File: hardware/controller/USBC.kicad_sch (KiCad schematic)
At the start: 1 part, among them J1 Joystick

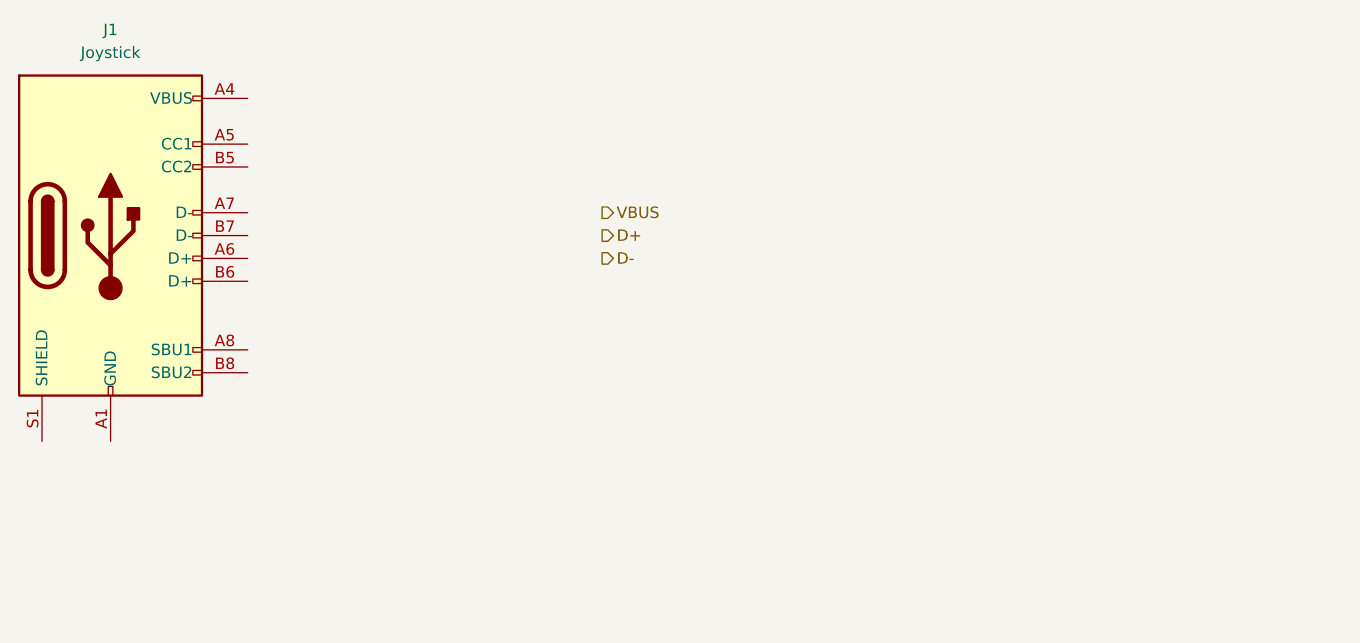
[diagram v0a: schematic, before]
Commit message: a
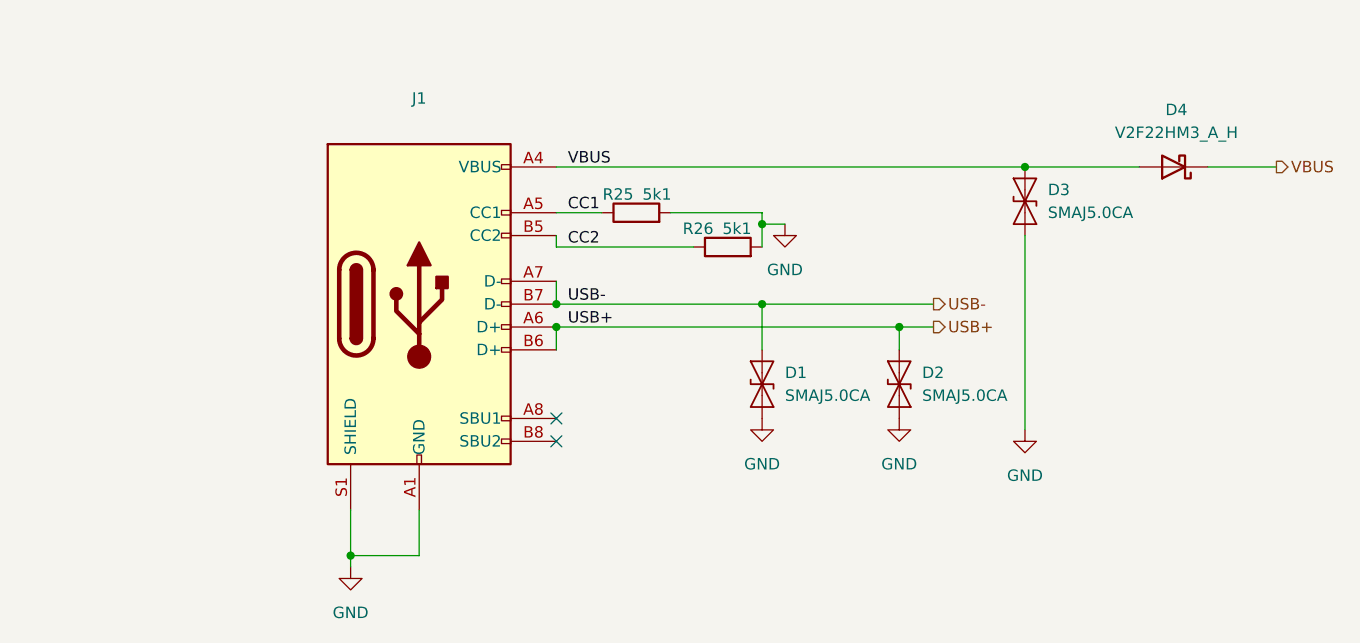
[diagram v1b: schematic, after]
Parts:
- added D1, D2, D3: SMAJ5.0CA, Diode_SMD:Infineon_SG-WLL-2-3_0.58x0.28_P0.36mm, symbol Diode:ESD131-B1-W0201
- added D4: V2F22HM3_A_H, Diode_SMD:D_SMA, symbol Diode:SS3150
- added R25, R26: 5k1, symbol Device:R
- J1: value Joystick -> ~
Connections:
- net VBUS: now also J1.A4 (VBUS), J1.A9 (VBUS), J1.B4 (VBUS), J1.B9 (VBUS), D3.2 (A2), D4.1 (K), D4.2 (A)
- net GND: now reaches J1.A1 (GND), J1.A12 (GND), J1.B1 (GND), J1.B12 (GND)
- net GND: now also J1.S1 (SHIELD), D1.1 (A1), D2.1 (A1), D3.1 (A1), R25.2, R26.2
- net CC1: now reaches J1.A5 (CC1)
- net CC1: now also R25.1
- net USB+: now reaches J1.A6 (D+)
- net USB+: now also J1.B6 (D+), D2.2 (A2)
- net USB-: now reaches J1.A7 (D-)
- net USB-: now also J1.B7 (D-), D1.2 (A2)
- net CC2: now reaches J1.B5 (CC2)
- net CC2: now also R26.1
- no-connect marks 0 -> 2
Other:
- moved on the sheet: J1
